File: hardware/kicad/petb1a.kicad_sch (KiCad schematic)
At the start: 31 parts, among them J1 TYPEC-304-ACP16, J2 DNP, J3 DNP, SW1 TD-1183SA-1.5H-250, SW2 TD-1183SA-1.5H-250, U1 USBLC6-2P6, U2 ESP32-S3-WROOM-1, U3 XC6220B331MR-G

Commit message: update pcb
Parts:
- J2, J3: footprint Connector_PinHeader_2.54mm:PinHeader_1x22_P2.54mm_Vertical -> petb1a:PinHeader_1x22_P2.54mm_Vertical
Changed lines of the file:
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@@
       (effects (font (size 1.27 1.27)) (justify left))
     )
-    (property "Footprint" "Connector_PinHeader_2.54mm:PinHeader_1x22_P2.54mm_Vertical" (at 194.31 112.395 0)
+    (property "Footprint" "petb1a:PinHeader_1x22_P2.54mm_Vertical" (at 194.31 112.395 0)
       (effects (font (size 1.27 1.27)) hide)
     )
@@
       (effects (font (size 1.27 1.27)) (justify left))
     )
-    (property "Footprint" "Connector_PinHeader_2.54mm:PinHeader_1x22_P2.54mm_Vertical" (at 181.61 112.395 0)
-      (effects (font (size 1.27 1.27)) hide)
-    )
+    (property "Footprint" "petb1a:PinHeader_1x22_P2.54mm_Vertical" (at 181.61 112.395 0)
+      (effects (font (size 1.27 1.27)) hide)
+    )

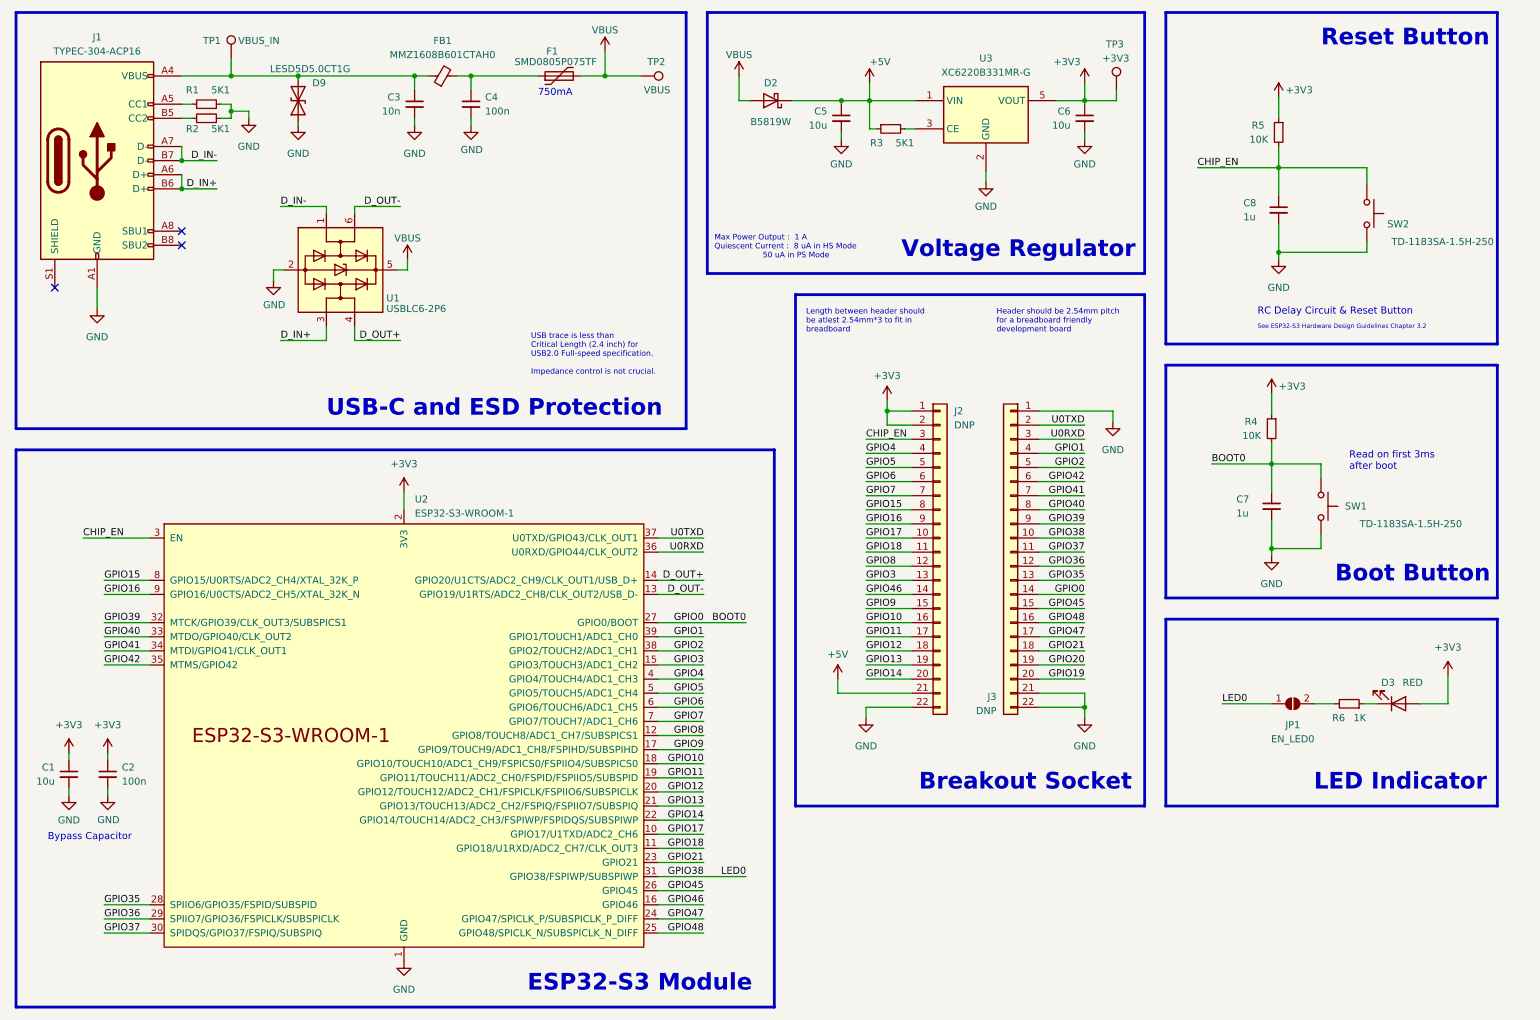
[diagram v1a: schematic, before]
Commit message: update board
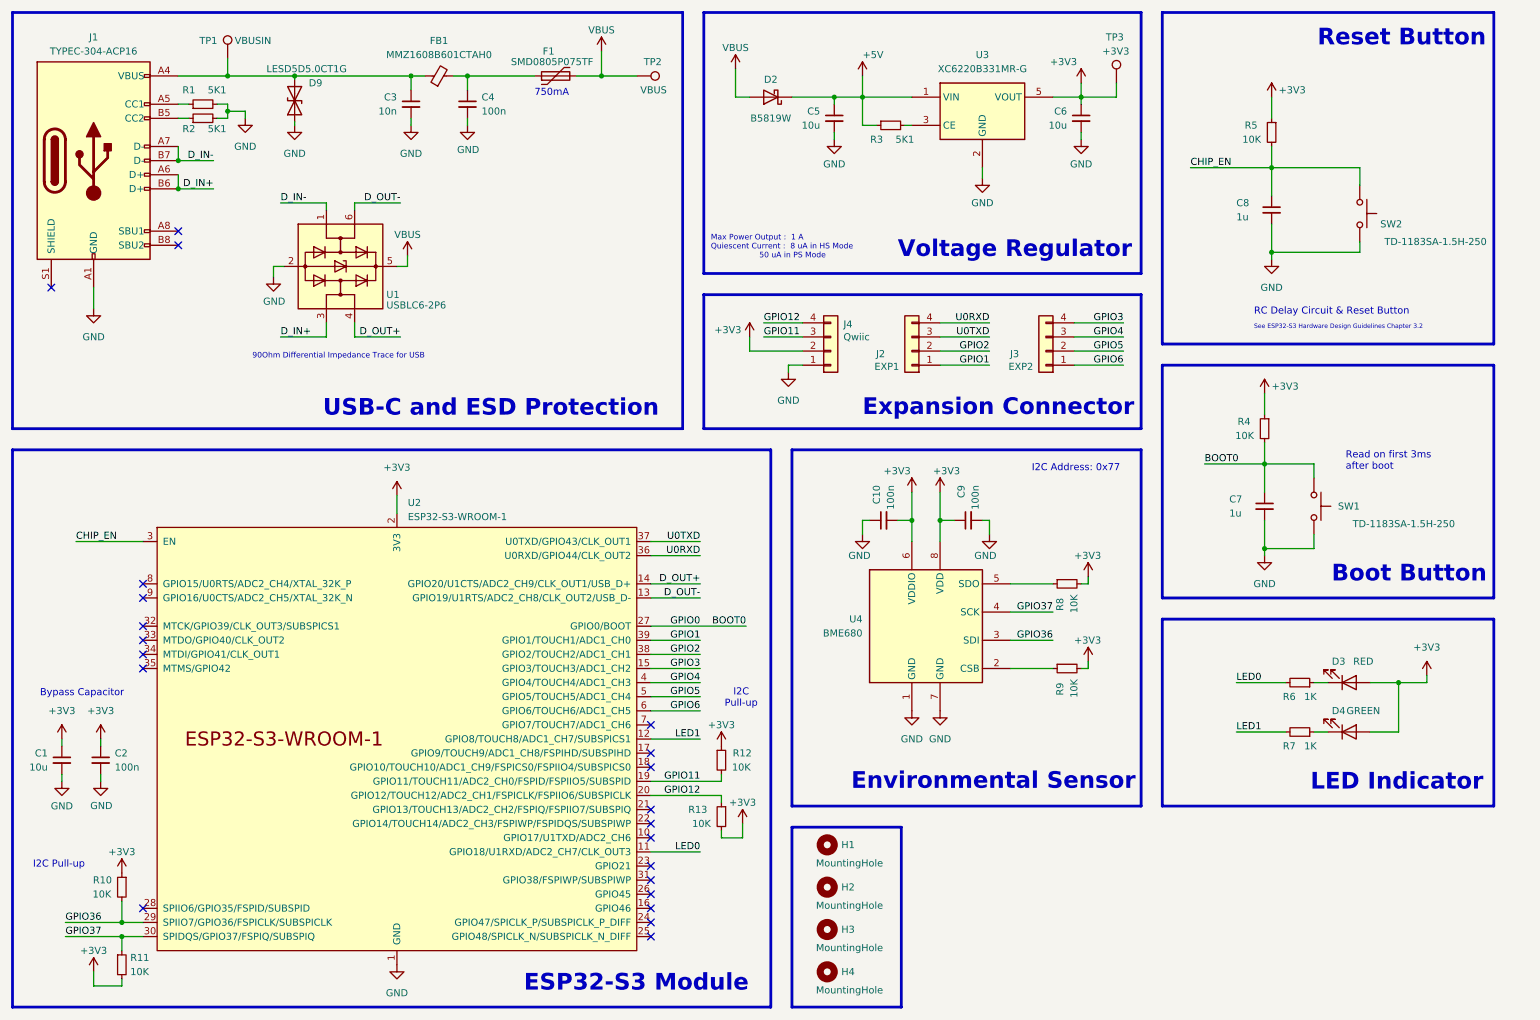
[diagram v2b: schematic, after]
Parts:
- removed J2, J3: DNP, petb1a:PinHeader_1x22_P2.54mm_Vertical, symbol Connector_Generic:Conn_01x22
- removed JP1: EN_LED0, Jumper:SolderJumper-2_P1.3mm_Open_RoundedPad1.0x1.5mm, symbol Jumper:SolderJumper_2_Open
- added C10, C9: 100n, Capacitor_SMD:C_0402_1005Metric, symbol Device:C_Small
- added D4: GREEN, LED_SMD:LED_0603_1608Metric, symbol Device:LED
- added H1, H2, H3, H4: MountingHole, MountingHole:MountingHole_3.2mm_M3, symbol Mechanical:MountingHole
- added J2: EXP1, petb1a:JST_SH_SM04B-SRSS-TB_1x04-1MP_P1.00mm_Horizontal, symbol Connector_Generic:Conn_01x04
- added J3: EXP2, petb1a:JST_SH_SM04B-SRSS-TB_1x04-1MP_P1.00mm_Horizontal, symbol Connector_Generic:Conn_01x04
- added J4: Qwiic, petb1a:JST_SH_SM04B-SRSS-TB_1x04-1MP_P1.00mm_Horizontal, symbol Connector_Generic:Conn_01x04
- added R10, R11, R12, R13, R8, R9: 10K, Resistor_SMD:R_0402_1005Metric, symbol Device:R_Small
- added R7: 1K, Resistor_SMD:R_0603_1608Metric, symbol Device:R_Small
- added U4: BME680, petb1a:Bosch_LGA-8_3x3mm_P0.8mm_ClockwisePinNumbering, symbol Sensor:BME680
- TP1: value VBUS_IN -> VBUSIN
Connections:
- net GPIO18 is gone; now on net LED0: U2.11 (GPIO18/U1RXD/ADC2_CH7/CLK_OUT3)
- net +3V3: now also C10.2, C9.1, D4.2 (A), J4.2 (Pin_2), R10.1, R11.2, R12.1, R13.2, R8.2, R9.2, U4.6 (VDDIO), U4.8 (VDD)
- net GND: now also C10.1, C9.2, J4.1 (Pin_1), U4.1 (GND), U4.7 (GND)
- net GPIO1: now also J2.1 (Pin_1)
- net GPIO11: now also J4.3 (Pin_3), R12.2
- net GPIO12: now also J4.4 (Pin_4), R13.1
- net GPIO2: now also J2.2 (Pin_2)
- net GPIO3: now also J3.4 (Pin_4)
- net GPIO36: now also R10.2, U4.3 (SDI)
- net GPIO37: now also R11.1, U4.4 (SCK)
- net GPIO4: now also J3.3 (Pin_3)
- net GPIO5: now also J3.2 (Pin_2)
- net GPIO6: now also J3.1 (Pin_1)
- net U0RXD: now also J2.4 (Pin_4)
- net U0TXD: now also J2.3 (Pin_3)
- net LED0: now reaches R6.2
- net GPIO10: no longer names the net of U2.18 (GPIO10/TOUCH10/ADC1_CH9/FSPICS0/FSPIIO4/SUBSPICS0)
- net GPIO13: no longer names the net of U2.21 (GPIO13/TOUCH13/ADC2_CH2/FSPIQ/FSPIIO7/SUBSPIQ)
- net GPIO14: no longer names the net of U2.22 (GPIO14/TOUCH14/ADC2_CH3/FSPIWP/FSPIDQS/SUBSPIWP)
- net GPIO15: no longer names the net of U2.8 (GPIO15/U0RTS/ADC2_CH4/XTAL_32K_P)
- net GPIO16: no longer names the net of U2.9 (GPIO16/U0CTS/ADC2_CH5/XTAL_32K_N)
- net GPIO17: no longer names the net of U2.10 (GPIO17/U1TXD/ADC2_CH6)
- net GPIO21: no longer names the net of U2.23 (GPIO21)
- net GPIO35: no longer names the net of U2.28 (SPIIO6/GPIO35/FSPID/SUBSPID)
- net GPIO38: no longer names the net of U2.31 (GPIO38/FSPIWP/SUBSPIWP)
- net GPIO39: no longer names the net of U2.32 (MTCK/GPIO39/CLK_OUT3/SUBSPICS1)
- net GPIO40: no longer names the net of U2.33 (MTDO/GPIO40/CLK_OUT2)
- net GPIO41: no longer names the net of U2.34 (MTDI/GPIO41/CLK_OUT1)
- net GPIO42: no longer names the net of U2.35 (MTMS/GPIO42)
- net GPIO45: no longer names the net of U2.26 (GPIO45)
- net GPIO46: no longer names the net of U2.16 (GPIO46)
- net GPIO47: no longer names the net of U2.24 (GPIO47/SPICLK_P/SUBSPICLK_P_DIFF)
- net GPIO48: no longer names the net of U2.25 (GPIO48/SPICLK_N/SUBSPICLK_N_DIFF)
- net GPIO7: no longer names the net of U2.7 (GPIO7/TOUCH7/ADC1_CH6)
- net GPIO8 renamed LED1
- net LED1: now also R7.2
- net GPIO9: no longer names the net of U2.17 (GPIO9/TOUCH9/ADC1_CH8/FSPIHD/SUBSPIHD)
- new net: R8.1, U4.5 (SDO)
- new net: D4.1 (K), R7.1
- new net: R9.1, U4.2 (CSB)
- no-connect marks 3 -> 22
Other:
- note added: "90Ohm Differential Impedance Trace for USB"
- note added: "Environmental Sensor"
- note added: "Expansion Connector"
- note added: "I2C Address: 0x77"
- note added: "I2C Pull-up"
- note removed: "Breakout Socket"
- note removed: "Header should be 2.54mm pitch for a breadboard friendly development board"
- note removed: "Length between header should be atlest 2.54mm*3 to fit in breadboard"
- note removed: "USB trace is less than Critical Length (2.4 inch) for USB2.0 Full-speed specification. Impedance control is not crucial."
- moved on the sheet: C1, C2, C3, C4, C5, C6, C7, C8, D2, D3, D9, F1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
